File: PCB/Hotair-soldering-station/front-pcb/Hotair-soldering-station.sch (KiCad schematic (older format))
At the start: 57 parts, among them J2 main-board-conn, J3 hot_on, J4 solder_on, Q1 BC817, Q10 BC807, Q11 BC807, Q12 BC807, Q13 BC807, Q14 BC807, Q2 BC817, Q3 BC817, Q4 BC817, Q5 BC817, Q6 BC817, Q7 BC817, Q8 BC817, Q9 BC807, SW1 HOTAIR_UP, SW2 HOTAIR_DOWN, SW3 SIRON_UP, SW4 SIRON_DOWN, SW5 SIRON_UP, SW6 SIRON_DOWN, U1 74HC595D, U2 74HC595D, U3 My-Footprints:3-digit-7-segme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, U4 3-dig-7-seg-display-common-an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

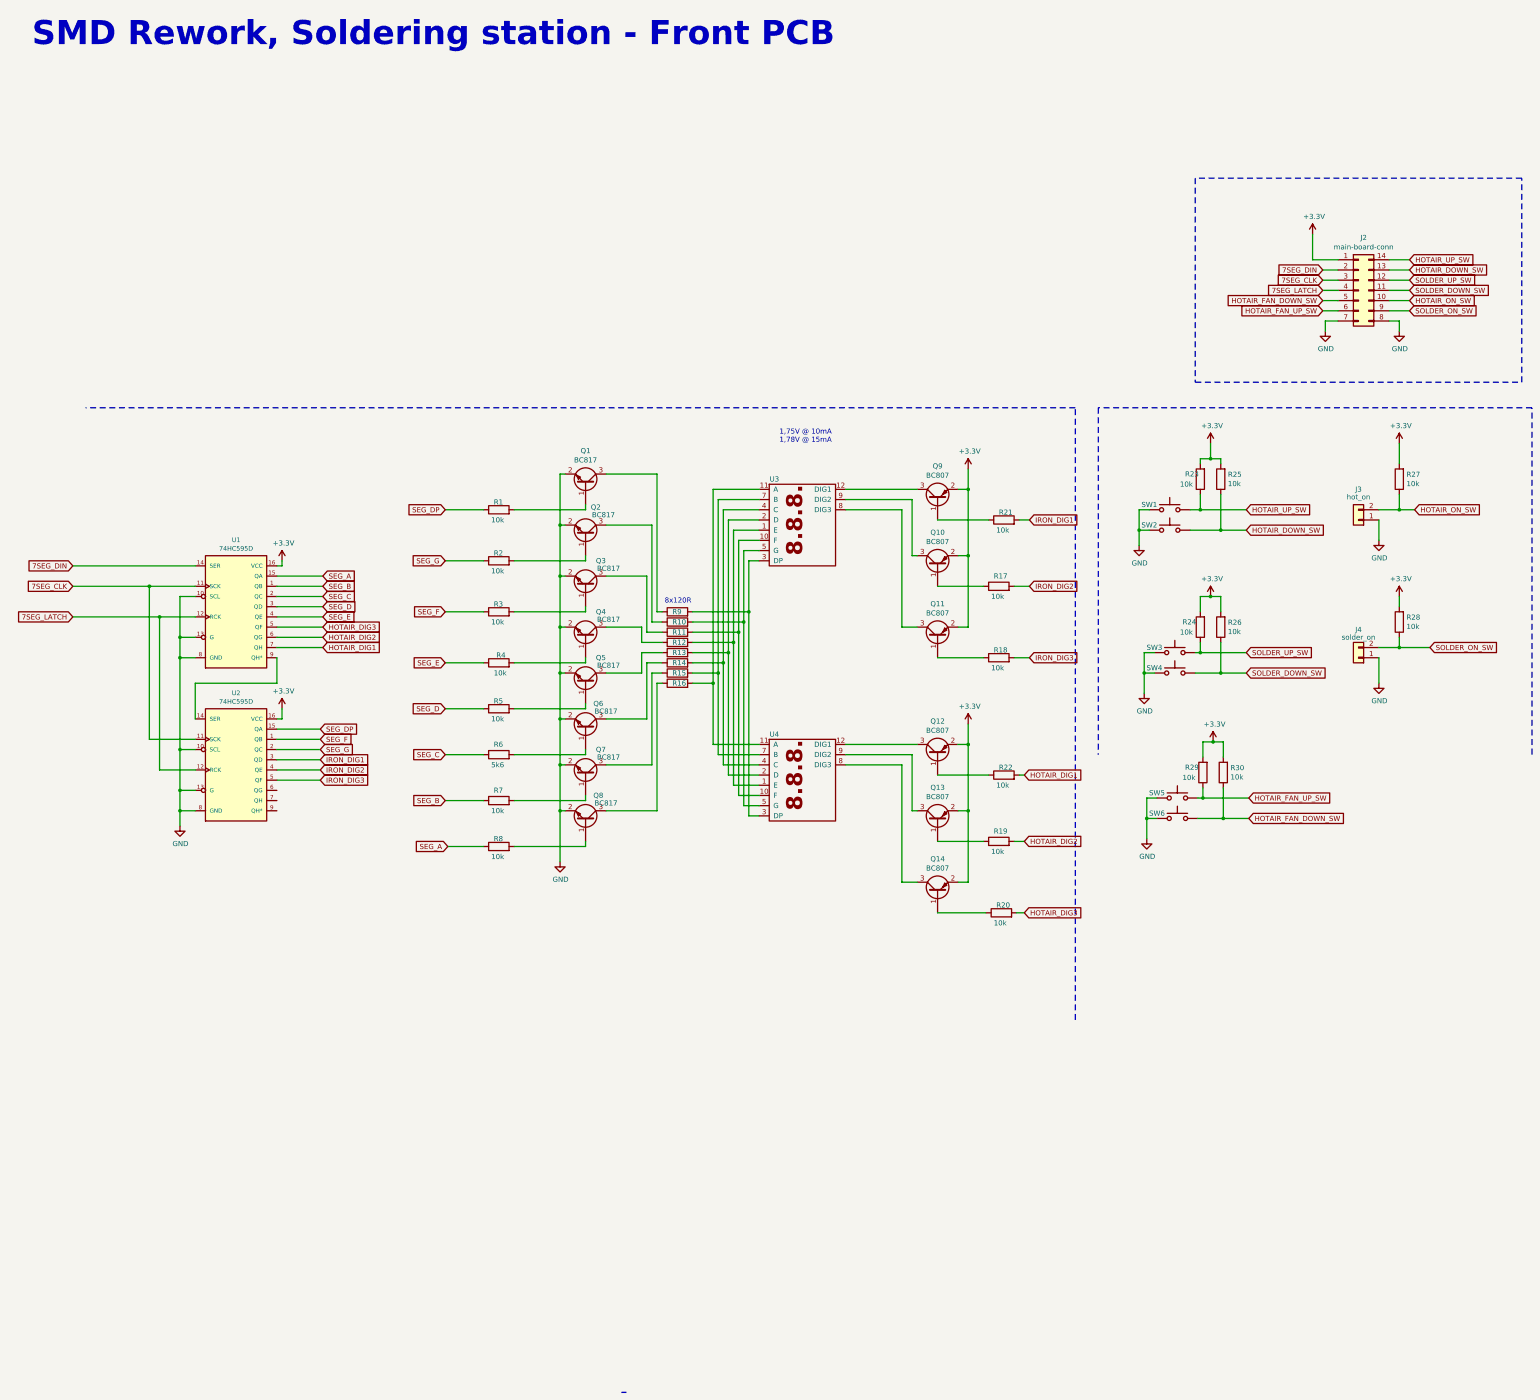
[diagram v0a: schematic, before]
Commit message: front PCB - finish
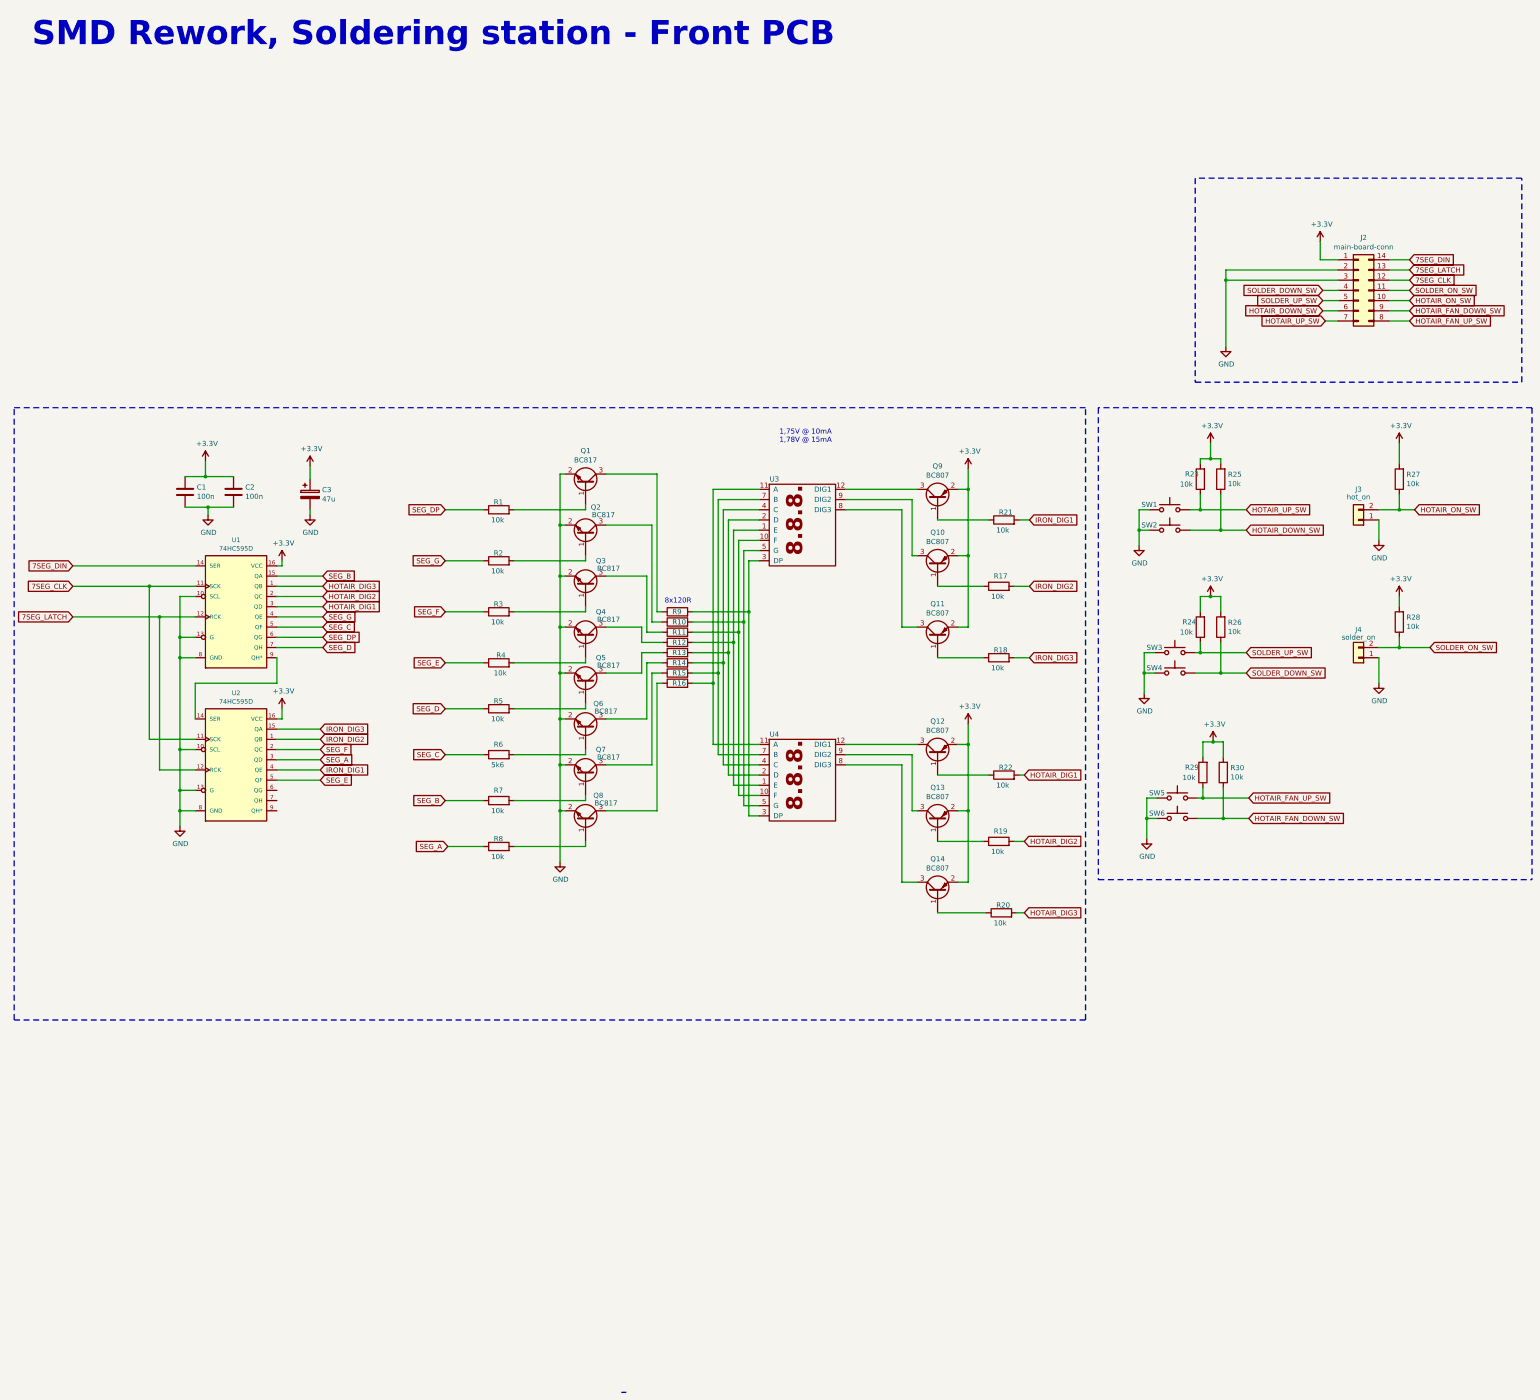
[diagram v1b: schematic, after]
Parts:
- added C1, C2: 100n, Capacitors:0805, symbol Device:C
- added C3: 47u, Capacitor_Tantalum_SMD:CP_EIA-3528-21_Kemet-B, symbol Device:CP
- SW1, SW2, SW3, SW4: footprint My-Footprints:push_button_12mm -> Switches:TACTILE_SWITCH_PTH_12MM
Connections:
- net +3V3: now also C1.1, C2.1, C3.1
- net 7SEG_CLK: now also J2.12 (Pin_12); no longer J2.3 (Pin_3)
- net 7SEG_DIN: now also J2.14 (Pin_14); no longer J2.2 (Pin_2)
- net 7SEG_LATCH: now also J2.13 (Pin_13); no longer J2.4 (Pin_4)
- net GND: now also J2.2 (Pin_2), J2.3 (Pin_3), C1.2, C2.2, C3.2; no longer J2.7 (Pin_7), J2.8 (Pin_8)
- net HOTAIR_DIG1: now also U1.3 (QD); no longer U1.7 (QH)
- net HOTAIR_DIG2: now also U1.2 (QC); no longer U1.6 (QG)
- net HOTAIR_DIG3: now also U1.1 (QB); no longer U1.5 (QF)
- net HOTAIR_DOWN_SW: now also J2.6 (Pin_6); no longer J2.13 (Pin_13)
- net HOTAIR_FAN_DOWN_SW: now also J2.9 (Pin_9); no longer J2.5 (Pin_5)
- net HOTAIR_FAN_UP_SW: now also J2.8 (Pin_8); no longer J2.6 (Pin_6)
- net HOTAIR_UP_SW: now also J2.7 (Pin_7); no longer J2.14 (Pin_14)
- net IRON_DIG1: now also U2.4 (QE); no longer U2.3 (QD)
- net IRON_DIG2: now also U2.1 (QB); no longer U2.4 (QE)
- net IRON_DIG3: now also U2.15 (QA); no longer U2.5 (QF)
- net SEG_A: now also U2.3 (QD); no longer U1.15 (QA)
- net SEG_B: now also U1.15 (QA); no longer U1.1 (QB)
- net SEG_C: now also U1.5 (QF); no longer U1.2 (QC)
- net SEG_D: now also U1.7 (QH); no longer U1.3 (QD)
- net SEG_DP: now also U1.6 (QG); no longer U2.15 (QA)
- net SEG_E: now also U2.5 (QF); no longer U1.4 (QE)
- net SEG_F: now also U2.2 (QC); no longer U2.1 (QB)
- net SEG_G: now also U1.4 (QE); no longer U2.2 (QC)
- net SOLDER_DOWN_SW: now also J2.4 (Pin_4); no longer J2.11 (Pin_11)
- net SOLDER_ON_SW: now also J2.11 (Pin_11); no longer J2.9 (Pin_9)
- net SOLDER_UP_SW: now also J2.5 (Pin_5); no longer J2.12 (Pin_12)
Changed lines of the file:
@@
 F 0 "SW1" H 11925 5775 50  0000 C CNN
 F 1 "HOTAIR_UP" H 12125 5919 50  0001 C CNN
-F 2 "My-Footprints:push_button_12mm" H 12125 5925 50  0001 C CNN
+F 2 "Switches:TACTILE_SWITCH_PTH_12MM" H 12125 5925 50  0001 C CNN
 F 3 "~" H 12125 5925 50  0001 C CNN
 	1    12125 5725
@@
 F 0 "SW2" H 11925 5975 50  0000 C CNN
 F 1 "HOTAIR_DOWN" H 12125 6119 50  0001 C CNN
-F 2 "My-Footprints:push_button_12mm" H 12125 6125 50  0001 C CNN
+F 2 "Switches:TACTILE_SWITCH_PTH_12MM" H 12125 6125 50  0001 C CNN
 F 3 "~" H 12125 6125 50  0001 C CNN
 	1    12125 5925
@@
 F 0 "SW3" H 11975 7175 50  0000 C CNN
 F 1 "SIRON_UP" H 12175 7319 50  0001 C CNN
-F 2 "My-Footprints:push_button_12mm" H 12175 7325 50  0001 C CNN
+F 2 "Switches:TACTILE_SWITCH_PTH_12MM" H 12175 7325 50  0001 C CNN
 F 3 "~" H 12175 7325 50  0001 C CNN
 	1    12175 7125
@@
 F 0 "SW4" H 11975 7375 50  0000 C CNN
 F 1 "SIRON_DOWN" H 12175 7519 50  0001 C CNN
-F 2 "My-Footprints:push_button_12mm" H 12175 7525 50  0001 C CNN
+F 2 "Switches:TACTILE_SWITCH_PTH_12MM" H 12175 7525 50  0001 C CNN
 F 3 "~" H 12175 7525 50  0001 C CNN
 	1    12175 7325
@@
 SOLDER_ON_SW
 Wire Notes Line
-	15675 8125 15675 4725
-Wire Notes Line
 	15675 4725 11425 4725
-Wire Notes Line
-	11425 4725 11425 8125
 $Comp
 L Hotair-soldering-station-rescue:3-dig-7-seg-display-common-anode-My-Lib U4
@@
 	3800 8375 3375 8375
 Wire Notes Line
-	11200 10725 11200 4725
-Wire Notes Line
-	11200 4725 1500 4725
+	11300 10725 11300 4725
 $Comp
 L Connector_Generic:Conn_02x07_Counter_Clockwise J2
@@
 	1    0    0    -1
 $EndComp
-$Comp
-L power:GND #PWR0114
-U 1 1 5F81599D
-P 14375 3975
-F 0 "#PWR0114" H 14375 3725 50  0001 C CNN
-F 1 "GND" H 14380 3802 50  0000 C CNN
-F 2 "" H 14375 3975 50  0001 C CNN
-F 3 "" H 14375 3975 50  0001 C CNN
-	1    14375 3975
-	1    0    0    -1
-$EndComp
-Wire Wire Line
-	14275 3875 14375 3875
-Wire Wire Line
-	14375 3875 14375 3975
+Wire Wire Line
+	14275 3875 14475 3875
 $Comp
 L power:+3.3V #PWR0115
 U 1 1 5F82E9E7
-P 13525 3025
-F 0 "#PWR0115" H 13525 2875 50  0001 C CNN
-F 1 "+3.3V" H 13540 3198 50  0000 C CNN
-F 2 "" H 13525 3025 50  0001 C CNN
-F 3 "" H 13525 3025 50  0001 C CNN
-	1    13525 3025
-	1    0    0    -1
-$EndComp
-Wire Wire Line
-	13775 3275 13525 3275
-Wire Wire Line
-	13525 3275 13525 3025
-Text GLabel 14475 3275 2    50   Input ~ 0
+P 13600 3100
+F 0 "#PWR0115" H 13600 2950 50  0001 C CNN
+F 1 "+3.3V" H 13615 3273 50  0000 C CNN
+F 2 "" H 13600 3100 50  0001 C CNN
+F 3 "" H 13600 3100 50  0001 C CNN
+	1    13600 3100
+	1    0    0    -1
+$EndComp
+Text GLabel 13650 3875 0    50   Input ~ 0
 HOTAIR_UP_SW
-Text GLabel 14475 3375 2    50   Input ~ 0
+Text GLabel 13625 3775 0    50   Input ~ 0
 HOTAIR_DOWN_SW
-Text GLabel 14475 3475 2    50   Input ~ 0
+Text GLabel 13625 3675 0    50   Input ~ 0
 SOLDER_UP_SW
-Text GLabel 14475 3575 2    50   Input ~ 0
+Text GLabel 13625 3575 0    50   Input ~ 0
 SOLDER_DOWN_SW
 Text GLabel 14475 3675 2    50   Input ~ 0
 HOTAIR_ON_SW
-Text GLabel 14475 3775 2    50   Input ~ 0
+Text GLabel 14475 3575 2    50   Input ~ 0
 SOLDER_ON_SW
-Text GLabel 13625 3375 0    50   Input ~ 0
+Text GLabel 14475 3275 2    50   Input ~ 0
 7SEG_DIN
-Text GLabel 13625 3475 0    50   Input ~ 0
+Text GLabel 14475 3475 2    50   Input ~ 0
 7SEG_CLK
-Text GLabel 13625 3575 0    50   Input ~ 0
+Text GLabel 14475 3375 2    50   Input ~ 0
 7SEG_LATCH
-Wire Wire Line
-	13625 3375 13775 3375
-Wire Wire Line
-	13625 3475 13775 3475
 Wire Wire Line
 	13625 3575 13775 3575
@@
 Wire Wire Line
 	3825 7075 3375 7075
+Text GLabel 3800 8175 2    50   Input ~ 0
+SEG_A
 Text GLabel 3825 6375 2    50   Input ~ 0
-SEG_A
+SEG_B
+Text GLabel 3825 6875 2    50   Input ~ 0
+SEG_C
+Text GLabel 3825 7075 2    50   Input ~ 0
+SEG_D
+Text GLabel 3800 8375 2    50   Input ~ 0
+SEG_E
+Text GLabel 3800 8075 2    50   Input ~ 0
+SEG_F
+Text GLabel 3825 6775 2    50   Input ~ 0
+SEG_G
+Text GLabel 3825 6975 2    50   Input ~ 0
+SEG_DP
+Text GLabel 3825 6675 2    50   Input ~ 0
+HOTAIR_DIG1
+Text GLabel 3825 6575 2    50   Input ~ 0
+HOTAIR_DIG2
 Text GLabel 3825 6475 2    50   Input ~ 0
-SEG_B
-Text GLabel 3825 6575 2    50   Input ~ 0
-SEG_C
-Text GLabel 3825 6675 2    50   Input ~ 0
-SEG_D
-Text GLabel 3825 6775 2    50   Input ~ 0
-SEG_E
+HOTAIR_DIG3
+Text GLabel 3800 8275 2    50   Input ~ 0
+IRON_DIG1
 Text GLabel 3800 7975 2    50   Input ~ 0
-SEG_F
-Text GLabel 3800 8075 2    50   Input ~ 0
-SEG_G
+IRON_DIG2
 Text GLabel 3800 7875 2    50   Input ~ 0
-SEG_DP
-Text GLabel 3825 7075 2    50   Input ~ 0
-HOTAIR_DIG1
-Text GLabel 3825 6975 2    50   Input ~ 0
-HOTAIR_DIG2
-Text GLabel 3825 6875 2    50   Input ~ 0
-HOTAIR_DIG3
-Text GLabel 3800 8175 2    50   Input ~ 0
-IRON_DIG1
-Text GLabel 3800 8275 2    50   Input ~ 0
-IRON_DIG2
-Text GLabel 3800 8375 2    50   Input ~ 0
 IRON_DIG3
 Text GLabel 5050 9025 0    50   Input ~ 0
@@
 IRON_DIG3
 $Comp
-L Switch:SW_Push SW5
-U 1 1 5F8FF5F0
-P 12200 8550
-F 0 "SW5" H 12000 8600 50  0000 C CNN
-F 1 "SIRON_UP" H 12200 8744 50  0001 C CNN
-F 2 "Switches:TACTILE_SWITCH_PTH_12MM" H 12200 8750 50  0001 C CNN
-F 3 "~" H 12200 8750 50  0001 C CNN
-	1    12200 8550
-	1    0    0    -1
-$EndComp
-$Comp
-L Switch:SW_Push SW6
-U 1 1 5F8FF5F6
-P 12200 8750
-F 0 "SW6" H 12000 8800 50  0000 C CNN
-F 1 "SIRON_DOWN" H 12200 8944 50  0001 C CNN
-F 2 "Switches:TACTILE_SWITCH_PTH_12MM" H 12200 8950 50  0001 C CNN
-F 3 "~" H 12200 8950 50  0001 C CNN
-	1    12200 8750
-	1    0    0    -1
-$EndComp
-$Comp
 L power:GND #PWR0117
 U 1 1 5F8FF5FC
@@
 	12900 8750 12650 8750
 Connection ~ 12650 8750
-Text GLabel 13625 3775 0    50   Input ~ 0
+Text GLabel 14475 3875 2    50   Input ~ 0
 HOTAIR_FAN_UP_SW
-Text GLabel 13625 3675 0    50   Input ~ 0
+Text GLabel 14475 3775 2    50   Input ~ 0
 HOTAIR_FAN_DOWN_SW
 Wire Wire Line
@@
 Wire Wire Line
 	13775 3775 13625 3775
+Wire Wire Line
+	13650 3875 13775 3875
+$Comp
+L Device:C C1
+U 1 1 5FAD48E3
+P 2475 5550
+F 0 "C1" H 2590 5596 50  0000 L CNN
+F 1 "100n" H 2590 5505 50  0000 L CNN
+F 2 "Capacitors:0805" H 2513 5400 50  0001 C CNN
+F 3 "~" H 2475 5550 50  0001 C CNN
+	1    2475 5550
+	1    0    0    -1
+$EndComp
+$Comp
+L Device:C C2
+U 1 1 5FAD4D73
+P 2950 5550
+F 0 "C2" H 3065 5596 50  0000 L CNN
+F 1 "100n" H 3065 5505 50  0000 L CNN
+F 2 "Capacitors:0805" H 2988 5400 50  0001 C CNN
+F 3 "~" H 2950 5550 50  0001 C CNN
+	1    2950 5550
+	1    0    0    -1
+$EndComp
+$Comp
+L power:+3.3V #PWR0120
+U 1 1 5FAD5487
+P 2675 5250
+F 0 "#PWR0120" H 2675 5100 50  0001 C CNN
+F 1 "+3.3V" H 2690 5423 50  0000 C CNN
+F 2 "" H 2675 5250 50  0001 C CNN
+F 3 "" H 2675 5250 50  0001 C CNN
+	1    2675 5250
+	1    0    0    -1
+$EndComp
+Wire Wire Line
+	2675 5400 2675 5250
+Wire Wire Line
+	2475 5400 2675 5400
+Wire Wire Line
+	2950 5400 2675 5400
+Connection ~ 2675 5400
+$Comp
+L power:GND #PWR0121
+U 1 1 5FB17501
+P 2700 5775
+F 0 "#PWR0121" H 2700 5525 50  0001 C CNN
+F 1 "GND" H 2705 5602 50  0000 C CNN
+F 2 "" H 2700 5775 50  0001 C CNN
+F 3 "" H 2700 5775 50  0001 C CNN
+	1    2700 5775
+	1    0    0    -1
+$EndComp
+Wire Wire Line
+	2475 5700 2700 5700
+Wire Wire Line
+	2700 5700 2700 5775
+Wire Wire Line
+	2950 5700 2700 5700
+Connection ~ 2700 5700
+Wire Wire Line
+	13775 3275 13600 3275
+Wire Wire Line
+	13600 3100 13600 3275
+$Comp
+L power:GND #PWR0114
+U 1 1 5FBDEBF7
+P 12675 4125
+F 0 "#PWR0114" H 12675 3875 50  0001 C CNN
+F 1 "GND" H 12680 3952 50  0000 C CNN
+F 2 "" H 12675 4125 50  0001 C CNN
+F 3 "" H 12675 4125 50  0001 C CNN
+	1    12675 4125
+	1    0    0    -1
+$EndComp
+Wire Wire Line
+	12675 3475 12675 4125
+Wire Wire Line
+	12675 3475 13775 3475
+Wire Wire Line
+	12675 3375 12675 3475
+Wire Wire Line
+	12675 3375 13775 3375
+Connection ~ 12675 3475
+$Comp
+L Switch:SW_Push SW6
+U 1 1 5F8FF5F6
+P 12200 8750
+F 0 "SW6" H 12000 8800 50  0000 C CNN
+F 1 "SIRON_DOWN" H 12200 8944 50  0001 C CNN
+F 2 "Switches:TACTILE_SWITCH_PTH_12MM" H 12200 8950 50  0001 C CNN
+F 3 "~" H 12200 8950 50  0001 C CNN
+	1    12200 8750
+	1    0    0    -1
+$EndComp
+$Comp
+L Switch:SW_Push SW5
+U 1 1 5F8FF5F0
+P 12200 8550
+F 0 "SW5" H 12000 8600 50  0000 C CNN
+F 1 "SIRON_UP" H 12200 8744 50  0001 C CNN
+F 2 "Switches:TACTILE_SWITCH_PTH_12MM" H 12200 8750 50  0001 C CNN
+F 3 "~" H 12200 8750 50  0001 C CNN
+	1    12200 8550
+	1    0    0    -1
+$EndComp
+Wire Notes Line
+	11300 10725 800  10725
+Wire Notes Line
+	800  10725 800  4725
+Wire Notes Line
+	800  4725 11300 4725
+Wire Notes Line
+	11425 9350 15675 9350
+Wire Notes Line
+	15675 4725 15675 9350
+Wire Notes Line
+	11425 4725 11425 9350
+$Comp
+L Device:CP C3
+U 1 1 5FCA1084
+P 3700 5575
+F 0 "C3" H 3818 5621 50  0000 L CNN
+F 1 "47u" H 3818 5530 50  0000 L CNN
+F 2 "Capacitor_Tantalum_SMD:CP_EIA-3528-21_Kemet-B" H 3738 5425 50  0001 C CNN
+F 3 "~" H 3700 5575 50  0001 C CNN
+	1    3700 5575
+	1    0    0    -1
+$EndComp
 $Comp
 L power:GND #PWR0119
-U 1 1 5F953902
-P 13650 3975
-F 0 "#PWR0119" H 13650 3725 50  0001 C CNN
-F 1 "GND" H 13655 3802 50  0000 C CNN
-F 2 "" H 13650 3975 50  0001 C CNN
-F 3 "" H 13650 3975 50  0001 C CNN
-	1    13650 3975
-	1    0    0    -1
-$EndComp
-Wire Wire Line
-	13650 3975 13650 3875
-Wire Wire Line
-	13650 3875 13775 3875
+U 1 1 5FCA17DE
+P 3700 5775
+F 0 "#PWR0119" H 3700 5525 50  0001 C CNN
+F 1 "GND" H 3705 5602 50  0000 C CNN
+F 2 "" H 3700 5775 50  0001 C CNN
+F 3 "" H 3700 5775 50  0001 C CNN
+	1    3700 5775
+	1    0    0    -1
+$EndComp
+$Comp
+L power:+3.3V #PWR0122
+U 1 1 5FCA1ABE
+P 3700 5300
+F 0 "#PWR0122" H 3700 5150 50  0001 C CNN
+F 1 "+3.3V" H 3715 5473 50  0000 C CNN
+F 2 "" H 3700 5300 50  0001 C CNN
+F 3 "" H 3700 5300 50  0001 C CNN
+	1    3700 5300
+	1    0    0    -1
+$EndComp
+Wire Wire Line
+	3700 5300 3700 5425
+Wire Wire Line
+	3700 5725 3700 5775
 $EndSCHEMATC
